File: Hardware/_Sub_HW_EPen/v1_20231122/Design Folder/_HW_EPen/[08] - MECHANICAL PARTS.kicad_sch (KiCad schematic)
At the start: 7 parts

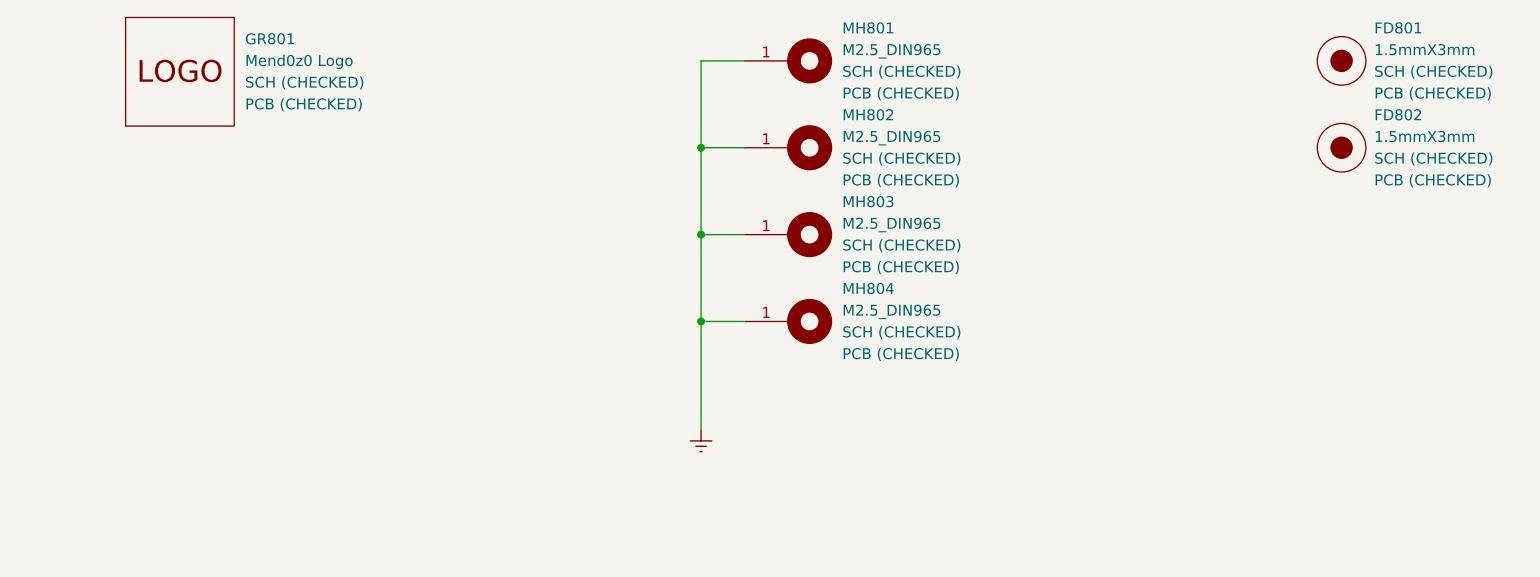
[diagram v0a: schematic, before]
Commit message: Updating file templates and structures...
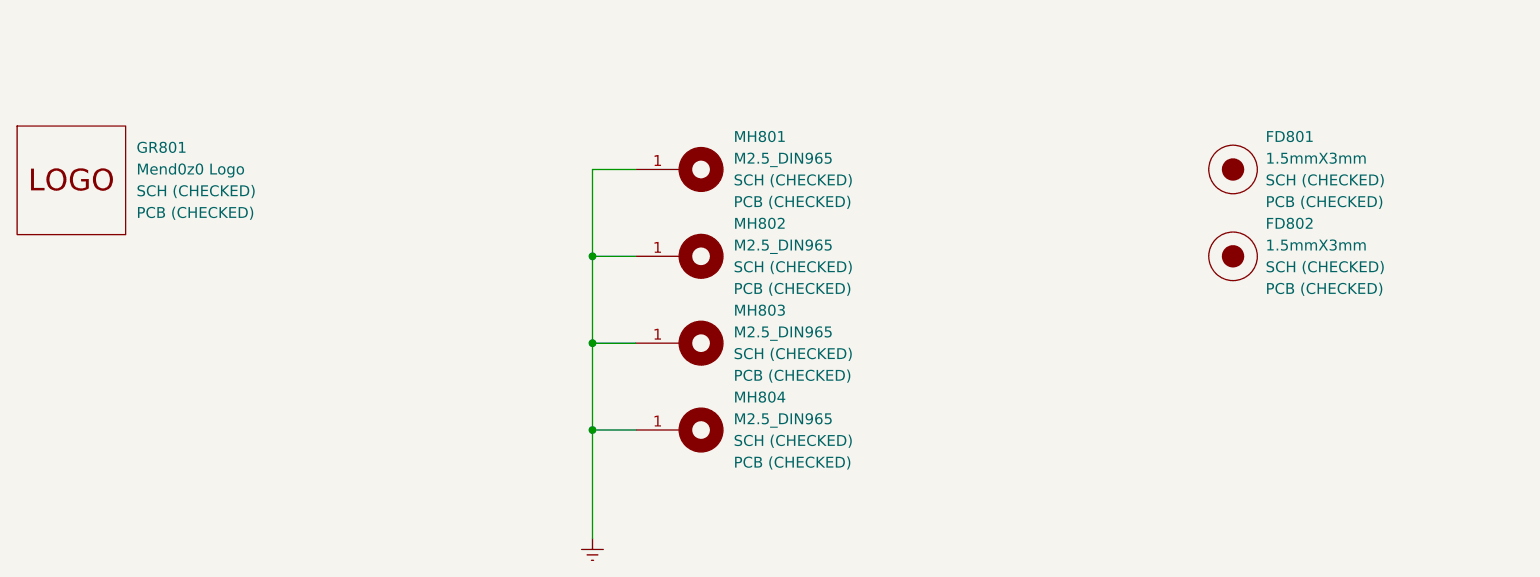
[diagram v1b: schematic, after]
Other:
- moved on the sheet: FD801, FD802, GR801, MH801, MH802, MH803, MH804
